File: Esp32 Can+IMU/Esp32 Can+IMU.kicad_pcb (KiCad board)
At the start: 2 copper layers, 57 x 62 mm, 86 parts, among them J1 Conn_01x04_Pin, J11 Qwiic_Vertical, J12 USB_C_Receptacle_USB2.0_16P, J2 Conn_01x04_Pin, J4 PINHD_1x3_Male, J5 PINHD_1x3_Male, J6 PINHD_1x3_Male, J7 PINHD_1x3_Male, J8 PINHD_1x3_Male, J9 PINHD_1x3_Male, SW1 SMD_4.2x3.2mm_h2.5mm, SW2 SMD_4.2x3.2mm_h2.5mm, U1 ESP32-S3-WROOM-1, U2 ISM6HG256XTR, U3 SN65HVD230DR, U4 TPS54360BQDDARQ1, U5 AP2112K-3.3, U6 USBLC6-2P6

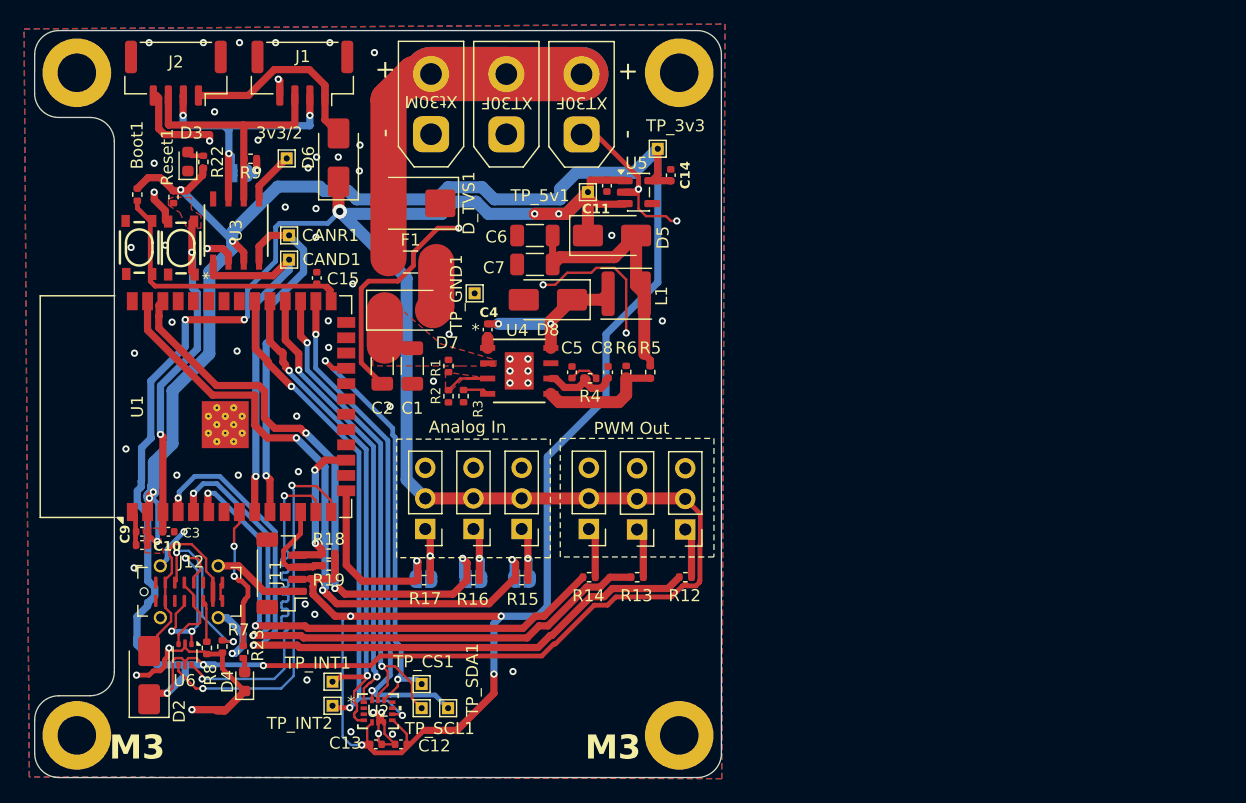
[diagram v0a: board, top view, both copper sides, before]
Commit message: Update ESP32 CAN IMU board revision
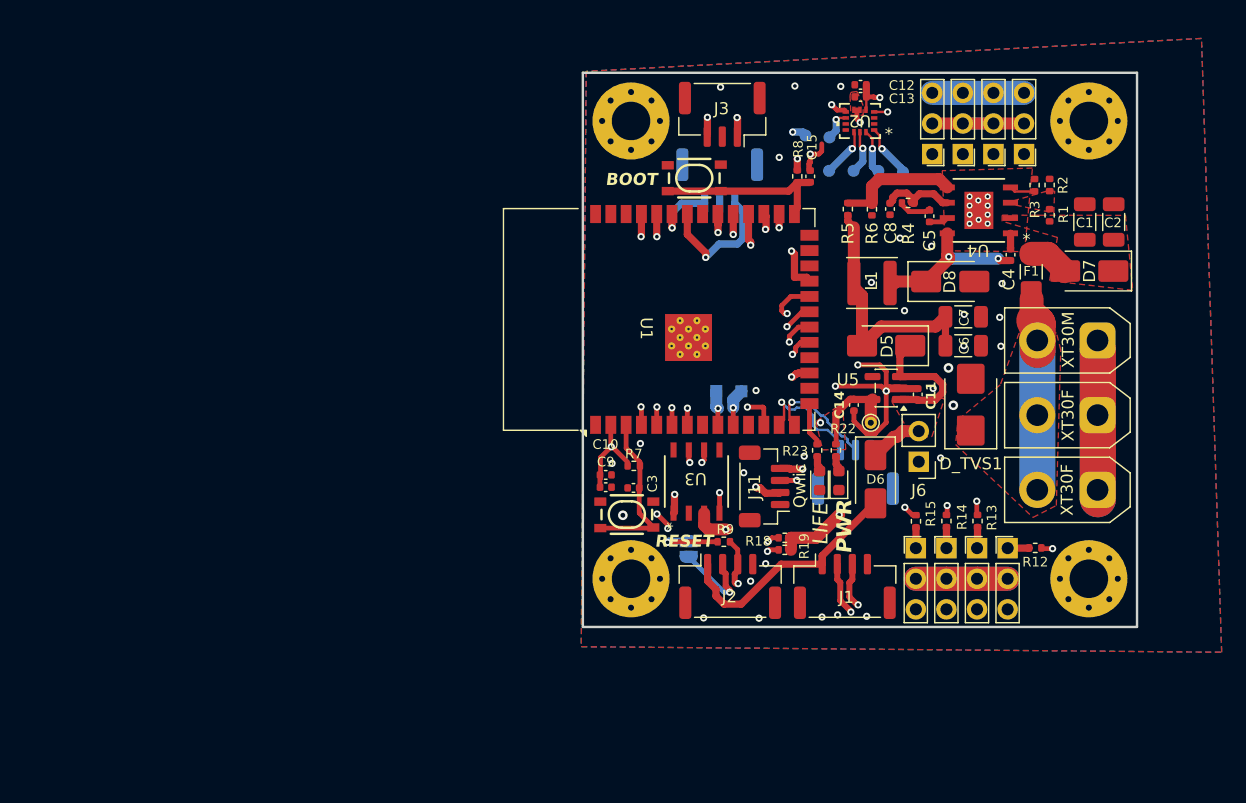
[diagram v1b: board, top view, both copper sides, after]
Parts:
- removed 3v3/2: CAN_VREF, TestPoint:TestPoint_THTPad_1.0x1.0mm_Drill0.5mm
- removed Boot1, R16, R17: 10kΩ, Resistor_SMD:R_0402_1005Metric
- removed D2: SS54, Diode_SMD:D_SMA
- removed JP2, JP3, JP4: 3v3 input, Jumper:SolderJumper-2_P1.3mm_Open_RoundedPad1.0x1.5mm
- removed SW1, SW2: SMD_4.2x3.2mm_h2.5mm, PCM_SparkFun-Switch:Push_SMD_4.2x3.2mm
- removed TP_5v1: 5v, TestPoint:TestPoint_THTPad_1.0x1.0mm_Drill0.5mm
- removed TP_GND1: GND, TestPoint:TestPoint_THTPad_1.0x1.0mm_Drill0.5mm
- removed U6: USBLC6-2P6, Package_TO_SOT_SMD:SOT-666
- added Boot2: BOOT, PCM_SparkFun-Switch:Push_SMD_4.2x3.2mm, F.Cu at (153.2, 72.8)
- added J10: PWM4, Connector:PinHeader_1x03_P2.54mm_Vertical_Close, F.Cu at (171.6, 103.5)
- added J13: ADC2, Connector:PinHeader_1x03_P2.54mm_Vertical_Close, F.Cu at (175.5, 70.8)
- added J14: ADC3, Connector:PinHeader_1x03_P2.54mm_Vertical_Close, F.Cu at (178.1, 70.8)
- added J15: ADC4, Connector:PinHeader_1x03_P2.54mm_Vertical_Close, F.Cu at (180.6, 70.8)
- added J3: UART0, Connector_JST:JST_GH_SM03B-GHS-TB_1x03-1MP_P1.25mm_Horizontal, F.Cu at (155.6, 67.5)
- added TP_SDO1: SDO, TestPoint:TestPoint_Pad_D1.0mm, B.Cu at (170.6, 72.2)
- C11: value 1µF 10V X5R -> 1uF 10V X5R
- C12, C13: value 100nf -> 100nF
- C14: value 4.7µF 10V X5R -> 4.7uF 10V X5R
- C15, C3: value 100 nF -> 100nF
- CAND1, CANR1: footprint TestPoint:TestPoint_THTPad_1.0x1.0mm_Drill0.5mm -> TestPoint:TestPoint_Pad_1.0x1.0mm; moved to B.Cu
- CAN_TERM1: value CAN_TERM -> CAN 120R
- D3: value Green -> PWR
- D4: value Red -> LIFE
- H1: value MountingHole -> M3; footprint MountingHole:MountingHole_3.2mm_M3_ISO7380_Pad -> MountingHole:MountingHole_3.2mm_M3_Pad_Via; moved to B.Cu
- H2, H3, H4: value MountingHole -> M3; footprint MountingHole:MountingHole_3.2mm_M3_ISO7380_Pad -> MountingHole:MountingHole_3.2mm_M3_Pad_Via
- J1: value Conn_01x04_Pin -> CAN0
- J11: value Qwiic_Vertical -> Qwiic
- J12: value USB_C_Receptacle_USB2.0_16P -> ADC1; footprint Connector_USB:USB_C_Receptacle_G-Switch_GT-USB-7051x -> Connector:PinHeader_1x03_P2.54mm_Vertical_Close
- J2: value Conn_01x04_Pin -> CAN1
- J4: value PINHD_1x3_Male -> UART1; footprint Connector_PinHeader_2.54mm:PinHeader_1x03_P2.54mm_Vertical -> Connector_JST:JST_GH_SM03B-GHS-TB_1x03-1MP_P1.25mm_Horizontal; moved to B.Cu
- J5: value PINHD_1x3_Male -> USB; footprint Connector_PinHeader_2.54mm:PinHeader_1x03_P2.54mm_Vertical -> Connector_JST:JST_GH_SM03B-GHS-TB_1x03-1MP_P1.25mm_Horizontal; moved to B.Cu
- J6: value PINHD_1x3_Male -> 5V ⏚; footprint Connector_PinHeader_2.54mm:PinHeader_1x03_P2.54mm_Vertical -> Connector_PinHeader_2.54mm:PinHeader_1x02_P2.54mm_Vertical
- J7: value PINHD_1x3_Male -> PWM1; footprint Connector_PinHeader_2.54mm:PinHeader_1x03_P2.54mm_Vertical -> Connector:PinHeader_1x03_P2.54mm_Vertical_Close
- J8: value PINHD_1x3_Male -> PWM2; footprint Connector_PinHeader_2.54mm:PinHeader_1x03_P2.54mm_Vertical -> Connector:PinHeader_1x03_P2.54mm_Vertical_Close
- J9: value PINHD_1x3_Male -> PWM3; footprint Connector_PinHeader_2.54mm:PinHeader_1x03_P2.54mm_Vertical -> Connector:PinHeader_1x03_P2.54mm_Vertical_Close
- R15: value 10kΩ -> 33Ω
- R7, R8: value 5.1kΩ -> 10k
- Reset1: value 10kΩ -> RESET; footprint Resistor_SMD:R_0402_1005Metric -> PCM_SparkFun-Switch:Push_SMD_4.2x3.2mm
- TP_3v3: footprint TestPoint:TestPoint_THTPad_1.0x1.0mm_Drill0.5mm -> TestPoint:TestPoint_THTPad_D1.0mm_Drill0.5mm
- TP_CS1: value IMU CS -> CS1; footprint TestPoint:TestPoint_THTPad_1.0x1.0mm_Drill0.5mm -> TestPoint:TestPoint_Pad_D1.0mm; moved to B.Cu
- TP_INT1: value IMU INT1 -> INT1; footprint TestPoint:TestPoint_THTPad_1.0x1.0mm_Drill0.5mm -> TestPoint:TestPoint_Pad_D1.0mm; moved to B.Cu
- TP_INT2: value IMU INT2 -> INT2; footprint TestPoint:TestPoint_THTPad_1.0x1.0mm_Drill0.5mm -> TestPoint:TestPoint_Pad_D1.0mm; moved to B.Cu
- TP_SCL1: value IMU SCL -> SCL1; footprint TestPoint:TestPoint_THTPad_1.0x1.0mm_Drill0.5mm -> TestPoint:TestPoint_Pad_D1.0mm; moved to B.Cu
- TP_SDA1: value IMU_SDA -> SDA1; footprint TestPoint:TestPoint_THTPad_1.0x1.0mm_Drill0.5mm -> TestPoint:TestPoint_Pad_D1.0mm; moved to B.Cu
- XT30F1, XT30F2: value Conn_01x02 -> XT30F
- XT30M1: value Conn_01x02 -> XT30M
- moved H4 93.9 mm to (186.0, 106.0), turned to -90 degrees
- moved J12 71.6 mm to (173.0, 70.8), turned to 180 degrees
- moved C13 67.1 mm to (167.1, 66.0), turned to 180 degrees
- moved C12 66.7 mm to (167.1, 65.0)
- moved U2 63.2 mm to (167.0, 68.0), turned to 180 degrees
- moved R8 62.7 mm to (161.8, 72.6), turned to 90 degrees
- moved J2 62.7 mm to (156.2, 106.6), turned to 0 degrees
- moved XT30F1 62.7 mm to (186.7, 98.6), turned to 180 degrees
- moved TP_INT2 62.7 mm to (164.5, 69.4), turned to -90 degrees
- moved J1 62.0 mm to (165.7, 106.6), turned to 0 degrees
- moved C2 61.9 mm to (188.1, 76.4), turned to 90 degrees
- moved D3 60.2 mm to (165.2, 97.8)
- moved TP_INT1 60.0 mm to (162.5, 69.2), turned to -90 degrees
- moved R22 57.7 mm to (165.0, 95.3), turned to 90 degrees
- moved TP_SCL1 57.2 mm to (166.5, 72.1), turned to -90 degrees
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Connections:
- net CANH renamed CAN+
- net CANL renamed CAN-
- D_TVS1 pad 1: GND -> Net-(D_TVS1-K)
- D_TVS1 pad 2: Net-(D_TVS1-A) -> GND
- F1 pad 1: Net-(D_TVS1-A) -> Net-(D_TVS1-K)
- J4 pad 1: Net-(JP2-B) -> UART1TX
- J4 pad 2: +5V -> GND
- J4 pad 3: GND -> UART1RX
- J5 pad 1: Net-(JP3-B) -> GND
- J5 pad 2: +5V -> USB_D+
- J5 pad 3: GND -> USB_D-
- J6 pad 1: Net-(JP4-B) -> GND
- R15 pad 1: ADC_1 -> PWM_4
- R15 pad 2: Net-(JP2-B) -> Net-(J10-Pad1)
- R23 pad 2: Net-(U1-IO15) -> Net-(U1-IO3)
- R7 pad 1: Net-(J12-CC1) -> +3.3V
- R7 pad 2: GND -> Net-(U1-EN)
- R8 pad 1: Net-(J12-CC2) -> Net-(U1-IO0)
- R8 pad 2: GND -> +3.3V
- Reset1 pad 1: +3.3V -> GND
- U1 pad 15: ADC_3 -> Net-(U1-IO3)
- U1 pad 19: unconnected-(U1-IO11-Pad19) -> PWM_4
- U1 pad 20: unconnected-(U1-IO12-Pad20) -> PWM_3
- U1 pad 21: unconnected-(U1-IO13-Pad21) -> PWM_2
- U1 pad 22: unconnected-(U1-IO14-Pad22) -> PWM_1
- U1 pad 34: unconnected-(U1-IO41-Pad34) -> UART1RX
- U1 pad 35: unconnected-(U1-IO42-Pad35) -> UART1TX
- U1 pad 36: unconnected-(U1-RXD0-Pad36) -> UART0RX
- U1 pad 37: unconnected-(U1-TXD0-Pad37) -> UART0TX
- U1 pad 38: AD2_1 -> unconnected-(U1-IO2-Pad38)
- U1 pad 39: ADC_1 -> unconnected-(U1-IO1-Pad39)
- U1 pad 4: PWM_1 -> ADC1_CH1
- U1 pad 5: PWM_2 -> ADC1_CH0
- U1 pad 6: PWM_3 -> ADC1_CH5
- U1 pad 7: unconnected-(U1-IO7-Pad7) -> ADC1_CH6
- U1 pad 8: Net-(U1-IO15) -> unconnected-(U1-IO15-Pad8)
- XT30F1 pad 2: Net-(D_TVS1-A) -> Net-(D_TVS1-K)
- XT30F2 pad 2: Net-(D_TVS1-A) -> Net-(D_TVS1-K)
- XT30M1 pad 2: Net-(D_TVS1-A) -> Net-(D_TVS1-K)
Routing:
- net +5V: track 208.0 -> 47.7 mm, vias 8 -> 0
- net ADC_1: track 54.6 -> 0.00 mm, vias 3 -> 0
- net AD2_1: track 48.8 -> 0.00 mm, vias 3 -> 0
- net Net-(D_TVS1-A): track 42.6 -> 0.00 mm
- net ADC1_CH0: track 0.00 -> 40.6 mm, vias 0 -> 1
- net ADC1_CH1: track 0.00 -> 40.4 mm, vias 0 -> 1
- net ADC1_CH6: track 0.00 -> 38.6 mm, vias 0 -> 1
- net ADC1_CH5: track 0.00 -> 37.7 mm, vias 0 -> 1
- net GND: track 111.2 -> 80.7 mm, vias 65 -> 47
- net SDA: track 43.1 -> 15.5 mm
- net SCL: track 41.9 -> 16.2 mm
- net INT2: track 45.1 -> 20.2 mm, vias 3 -> 2
- net PWM_1: track 60.5 -> 35.7 mm
- net PWM_2: track 52.6 -> 28.0 mm
- net USB_D+: track 31.7 -> 9.31 mm, vias 2 -> 1
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- added copper zone on F.Cu, net +5V
- added copper zone on In1.Cu, net GND
- added copper zone on In2.Cu, net GND
- added copper zone on F.Cu, net Net-(D_TVS1-K)
- removed copper zone on F.Cu, net Net-(U1-EN)
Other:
- board size 57 x 62 mm -> 46 x 46 mm
- copper layers 2 -> 4
- board text added: "IMU"
- board text added: "MONKE BRAIN V2"
- board text added: "S + ⏚"
- board text added: "S 3 ⏚"
- board text added: "SCL"
- board text added: "SDA"
- board text added: "T⏚R"
- board text added: "⏚+"
- board text added: "⏚+-"
- board text added: "⏚LH+"
- board text removed: "3V3 Max Analog In Enable"
- board text removed: "Analog In"
- board text removed: "C4"
- board text removed: "M3"
- board text removed: "PWM Out"
- board text removed: "R1"
- board text removed: "R2"
- board text removed: "XT30F"
- board text removed: "Xt30M"
